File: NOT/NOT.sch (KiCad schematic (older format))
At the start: 1 part

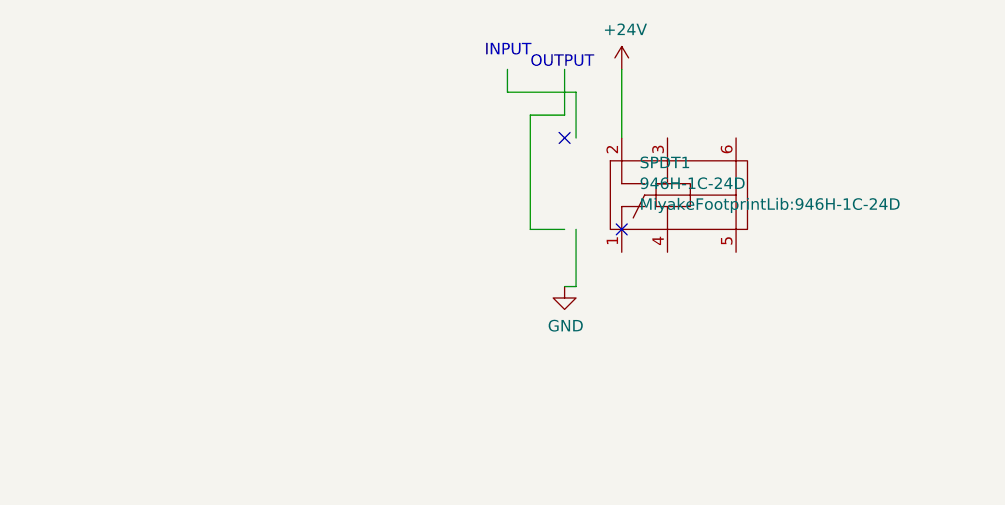
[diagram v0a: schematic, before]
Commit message: Add files via upload
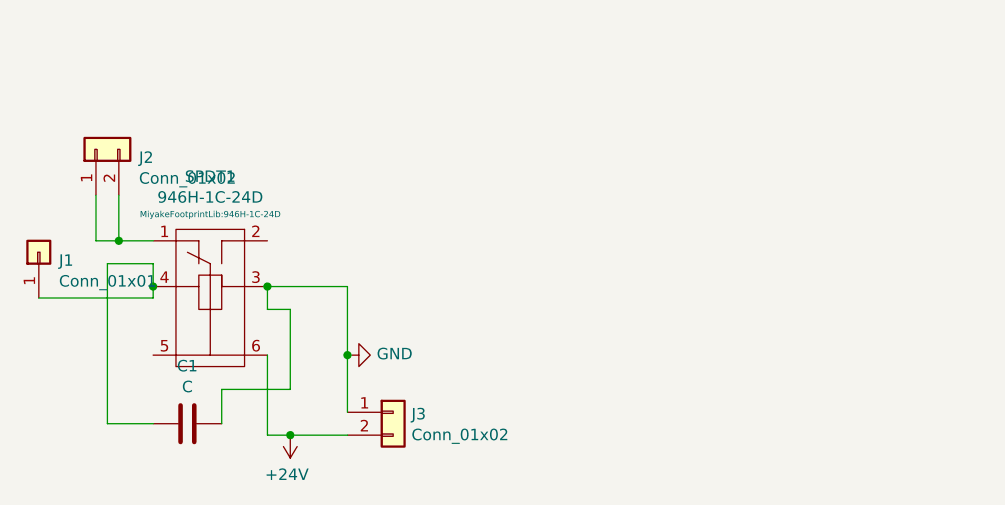
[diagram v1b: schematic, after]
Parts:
- added C1: C, MiyakeFootprintLib:Condensor, symbol Device:C
- added J1: Conn_01x01, Connector_PinHeader_2.54mm:PinHeader_1x01_P2.54mm_Vertical, symbol Connector_Generic:Conn_01x01
- added J2, J3: Conn_01x02, Connector_PinHeader_2.54mm:PinHeader_1x02_P2.54mm_Vertical, symbol Connector_Generic:Conn_01x02
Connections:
- wire segments 10 -> 21
- no-connect marks 2 -> 0
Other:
- note removed: "INPUT"
- note removed: "OUTPUT"
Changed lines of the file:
@@
 $Comp
 L MiyakeLib:946H-1C-24D SPDT1
-U 1 1 5ED20BFD
-P 6000 4000
-F 0 "SPDT1" V 6091 3772 50  0000 R CNN
-F 1 "946H-1C-24D" V 6000 3772 50  0000 R CNN
-F 2 "MiyakeFootprintLib:946H-1C-24D" V 5909 3772 50  0000 R CNN
-F 3 "" H 5950 4250 50  0001 C CNN
-	1    6000 4000
+U 1 1 5ED97C62
+P 4400 4100
+F 0 "SPDT1" H 4350 4231 50  0000 C CNN
+F 1 "946H-1C-24D" H 4350 4140 50  0000 C CNN
+F 2 "MiyakeFootprintLib:946H-1C-24D" H 4350 4066 27  0000 C CNN
+F 3 "" V 4350 3550 50  0001 C CNN
+	1    4400 4100
+	1    0    0    -1
+$EndComp
+$Comp
+L Connector_Generic:Conn_01x01 J1
+U 1 1 5ED99F3A
+P 3600 4300
+F 0 "J1" V 3564 4212 50  0000 R CNN
+F 1 "Conn_01x01" V 3473 4212 50  0000 R CNN
+F 2 "Connector_PinHeader_2.54mm:PinHeader_1x01_P2.54mm_Vertical" H 3600 4300 50  0001 C CNN
+F 3 "~" H 3600 4300 50  0001 C CNN
+	1    3600 4300
 	0    -1   -1   0
 $EndComp
 $Comp
-L power:+24V #PWR02
-U 1 1 5ED21C3E
-P 6150 3500
-F 0 "#PWR02" H 6150 3350 50  0001 C CNN
-F 1 "+24V" H 6165 3673 50  0000 C CNN
-F 2 "" H 6150 3500 50  0001 C CNN
-F 3 "" H 6150 3500 50  0001 C CNN
-	1    6150 3500
+L Connector_Generic:Conn_01x02 J2
+U 1 1 5ED9A3C0
+P 3850 3850
+F 0 "J2" V 3814 3662 50  0000 R CNN
+F 1 "Conn_01x02" V 3723 3662 50  0000 R CNN
+F 2 "Connector_PinHeader_2.54mm:PinHeader_1x02_P2.54mm_Vertical" H 3850 3850 50  0001 C CNN
+F 3 "~" H 3850 3850 50  0001 C CNN
+	1    3850 3850
+	0    -1   -1   0
+$EndComp
+$Comp
+L Connector_Generic:Conn_01x02 J3
+U 1 1 5ED9AF2C
+P 5150 5000
+F 0 "J3" H 5230 4992 50  0000 L CNN
+F 1 "Conn_01x02" H 5230 4901 50  0000 L CNN
+F 2 "Connector_PinHeader_2.54mm:PinHeader_1x02_P2.54mm_Vertical" H 5150 5000 50  0001 C CNN
+F 3 "~" H 5150 5000 50  0001 C CNN
+	1    5150 5000
 	1    0    0    -1
 $EndComp
 Wire Wire Line
-	6150 3800 6150 3500
+	3600 4500 4100 4500
+Wire Wire Line
+	4100 4500 4100 4450
+Wire Wire Line
+	4100 4250 3950 4250
+Wire Wire Line
+	3950 4250 3950 4050
+Wire Wire Line
+	3950 4250 3850 4250
+Wire Wire Line
+	3850 4250 3850 4050
+Connection ~ 3950 4250
+Wire Wire Line
+	4600 4450 4950 4450
+Wire Wire Line
+	4950 4450 4950 4750
+Wire Wire Line
+	4600 4750 4600 5100
+Wire Wire Line
+	4600 5100 4700 5100
 $Comp
-L power:GND #PWR01
-U 1 1 5ED22181
-P 5900 4450
-F 0 "#PWR01" H 5900 4200 50  0001 C CNN
-F 1 "GND" H 5905 4277 50  0000 C CNN
-F 2 "" H 5900 4450 50  0001 C CNN
-F 3 "" H 5900 4450 50  0001 C CNN
-	1    5900 4450
-	1    0    0    -1
+L power:GND #PWR02
+U 1 1 5ED9BA8D
+P 4950 4750
+F 0 "#PWR02" H 4950 4500 50  0001 C CNN
+F 1 "GND" V 4955 4622 50  0000 R CNN
+F 2 "" H 4950 4750 50  0001 C CNN
+F 3 "" H 4950 4750 50  0001 C CNN
+	1    4950 4750
+	0    -1   -1   0
+$EndComp
+Connection ~ 4950 4750
+Wire Wire Line
+	4950 4750 4950 5000
+$Comp
+L power:+24V #PWR01
+U 1 1 5ED9C200
+P 4700 5100
+F 0 "#PWR01" H 4700 4950 50  0001 C CNN
+F 1 "+24V" H 4715 5273 50  0000 C CNN
+F 2 "" H 4700 5100 50  0001 C CNN
+F 3 "" H 4700 5100 50  0001 C CNN
+	1    4700 5100
+	-1   0    0    1
+$EndComp
+Connection ~ 4700 5100
+Wire Wire Line
+	4700 5100 4950 5100
+$Comp
+L Device:C C1
+U 1 1 5ED9C8CA
+P 4250 5050
+F 0 "C1" V 3998 5050 50  0000 C CNN
+F 1 "C" V 4089 5050 50  0000 C CNN
+F 2 "MiyakeFootprintLib:Condensor" H 4288 4900 50  0001 C CNN
+F 3 "~" H 4250 5050 50  0001 C CNN
+	1    4250 5050
+	0    1    1    0
 $EndComp
 Wire Wire Line
-	5950 4200 5950 4450
+	4400 5050 4400 4900
 Wire Wire Line
-	5950 4450 5900 4450
+	4400 4900 4700 4900
 Wire Wire Line
-	5950 3800 5950 3600
+	4700 4900 4700 4550
 Wire Wire Line
-	5950 3600 5650 3600
+	4700 4550 4600 4550
 Wire Wire Line
-	5650 3600 5650 3500
-Text Notes 5550 3450 0    50   ~ 0
-INPUT
+	4600 4550 4600 4450
+Connection ~ 4600 4450
 Wire Wire Line
-	5900 4200 5750 4200
+	4100 5050 3900 5050
 Wire Wire Line
-	5750 4200 5750 3700
+	3900 5050 3900 4350
 Wire Wire Line
-	5750 3700 5900 3700
+	3900 4350 4100 4350
 Wire Wire Line
-	5900 3700 5900 3500
-Text Notes 5750 3500 0    50   ~ 0
-OUTPUT
-NoConn ~ 6150 4200
-NoConn ~ 5900 3800
+	4100 4350 4100 4450
+Connection ~ 4100 4450
 $EndSCHEMATC
